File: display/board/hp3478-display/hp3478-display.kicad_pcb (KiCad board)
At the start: 2 copper layers, 130.2 x 30.2 mm, 242 parts, among them J1 SFV10R-1ST, J2 DNP, U1 PIC16F15274-I/MP, U2 DNP

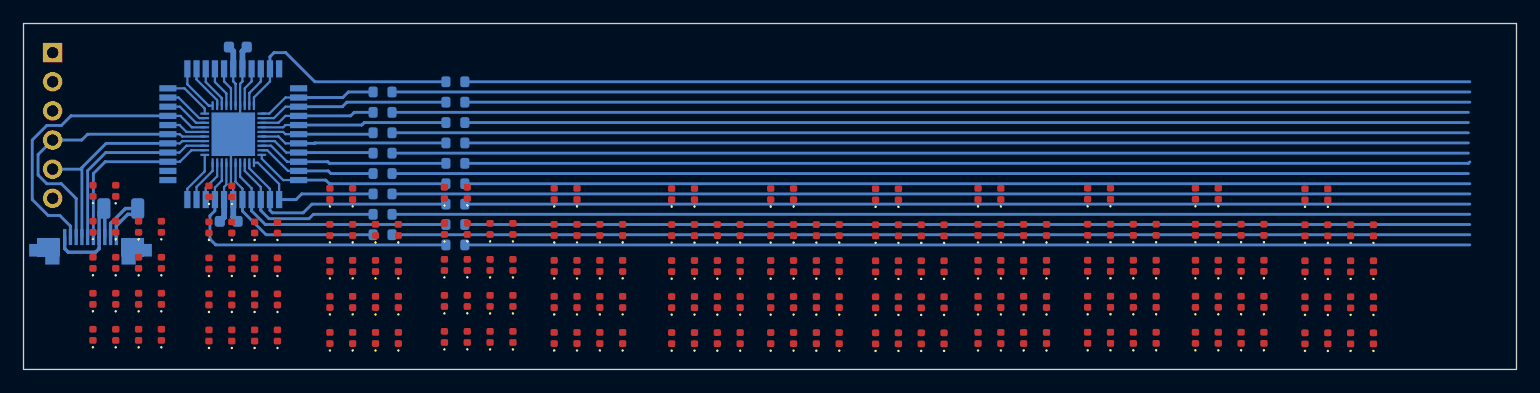
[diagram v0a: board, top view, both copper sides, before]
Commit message: Reorganize schematic.
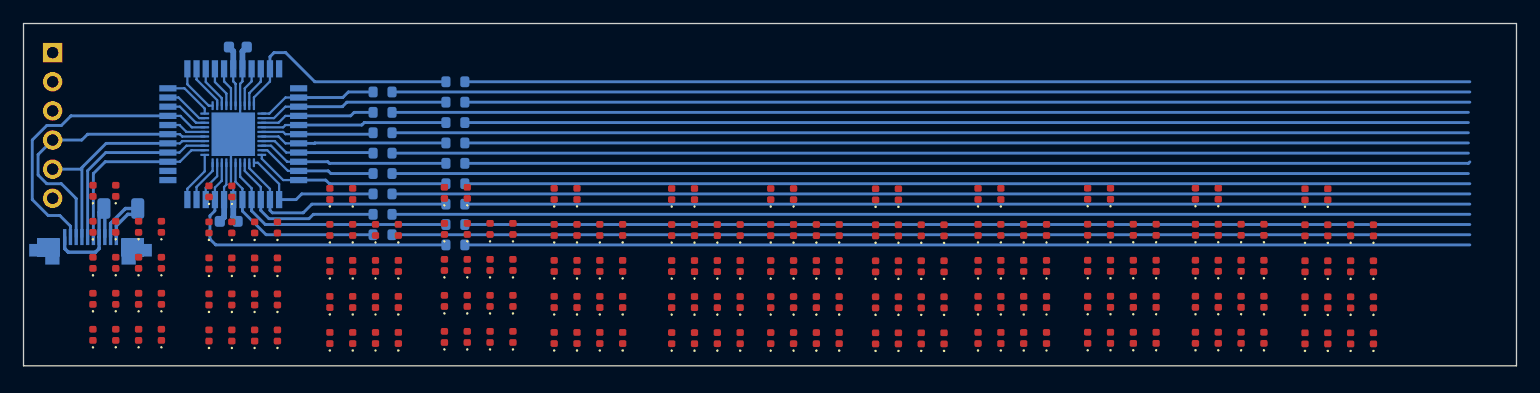
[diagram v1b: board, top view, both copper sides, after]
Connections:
- D1017 pad 1: /K8 -> Net-(D1018-Pad2)
- D1018 pad 2: /A16 -> Net-(D1018-Pad2)
- D1117 pad 1: /K9 -> Net-(D1118-Pad2)
- D1118 pad 2: /A16 -> Net-(D1118-Pad2)
- D1217 pad 1: /K10 -> Net-(D1218-Pad2)
- D1218 pad 2: /A16 -> Net-(D1218-Pad2)
- D1317 pad 1: /K11 -> Net-(D1318-Pad2)
- D1318 pad 2: /A16 -> Net-(D1318-Pad2)
- D217 pad 1: /K0 -> Net-(D218-Pad2)
- D218 pad 2: /A16 -> Net-(D218-Pad2)
- D317 pad 1: /K1 -> Net-(D318-Pad2)
- D318 pad 2: /A16 -> Net-(D318-Pad2)
- D417 pad 1: /K2 -> Net-(D418-Pad2)
- D418 pad 2: /A16 -> Net-(D418-Pad2)
- D517 pad 1: /K3 -> Net-(D518-Pad2)
- D518 pad 2: /A16 -> Net-(D518-Pad2)
- D617 pad 1: /K4 -> Net-(D618-Pad2)
- D618 pad 2: /A16 -> Net-(D618-Pad2)
- D717 pad 1: /K5 -> Net-(D718-Pad2)
- D718 pad 2: /A16 -> Net-(D718-Pad2)
- D817 pad 1: /K6 -> Net-(D818-Pad2)
- D818 pad 2: /A16 -> Net-(D818-Pad2)
- D917 pad 1: /K7 -> Net-(D918-Pad2)
- D918 pad 2: /A16 -> Net-(D918-Pad2)
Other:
- board size 130.2 x 30.2 mm -> 130.2 x 29.8 mm
